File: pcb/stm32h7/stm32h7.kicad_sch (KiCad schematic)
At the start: 39 parts, among them J6 Test Pads, SW1 SW_Push, SW2 SW_Push, SW3 SW_Push, U1 STM32H743VGTx, U11 TPS61169DCKR, U9 MT25QUxxxxxx1xW7, Y1 25MHz

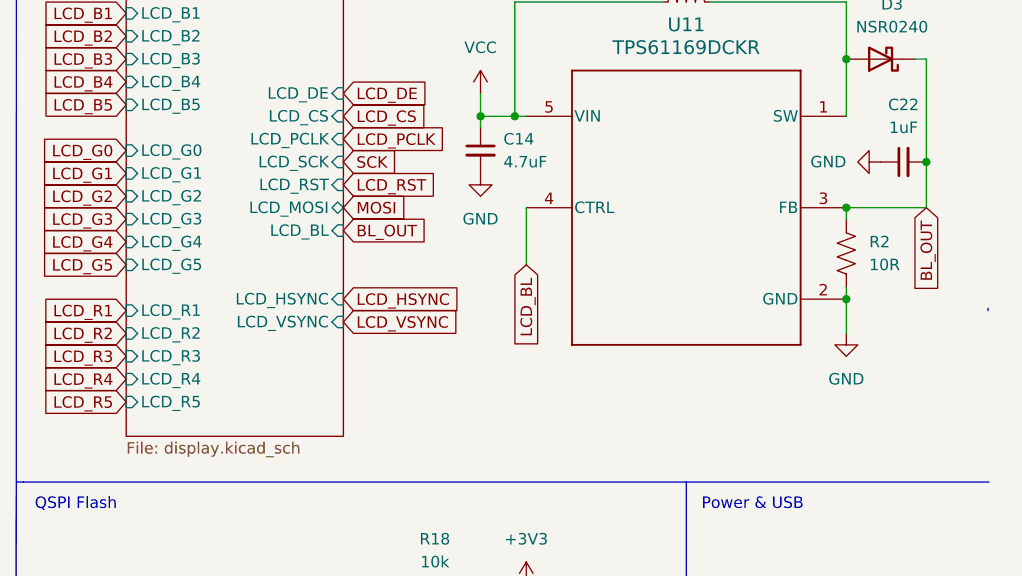
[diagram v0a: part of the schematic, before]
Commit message: fixed some wiring
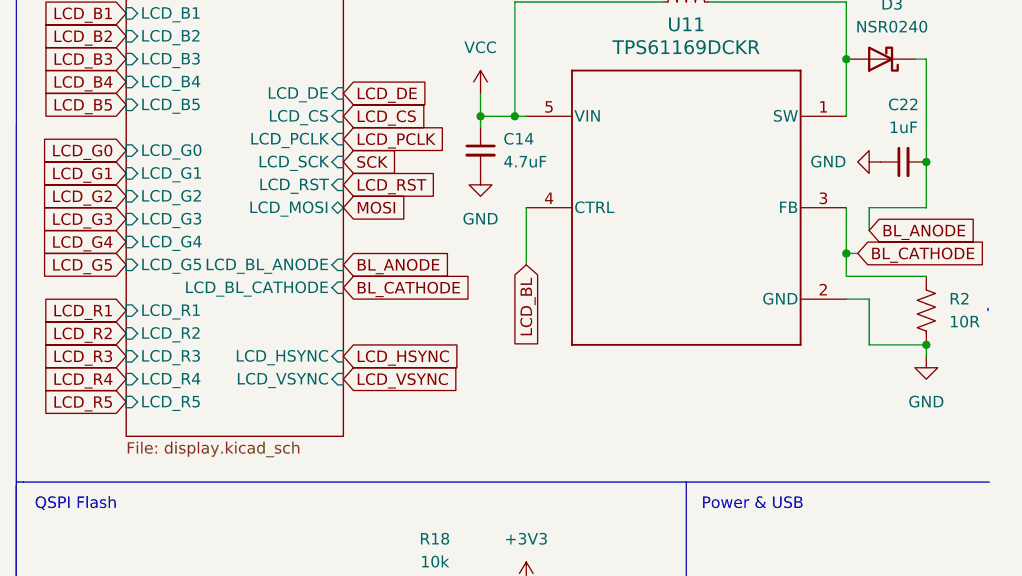
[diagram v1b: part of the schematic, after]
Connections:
- net GND: now also R2.1; no longer R2.2
- net BL_OUT renamed BL_ANODE
- net BL_ANODE: no longer R2.1, U11.3 (FB)
- new net BL_CATHODE: R2.2, U11.3 (FB)
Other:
- sheet LCD ports: added LCD_BL_ANODE, LCD_BL_CATHODE; removed LCD_BL
